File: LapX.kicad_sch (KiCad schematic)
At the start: 43 parts, among them J1 Conn_01x12, J2 Conn_02x01, J3 USB_C_Receptacle_PowerOnly_6P, J4 Micro_SD_Card_Det2, U2 TCMT4100

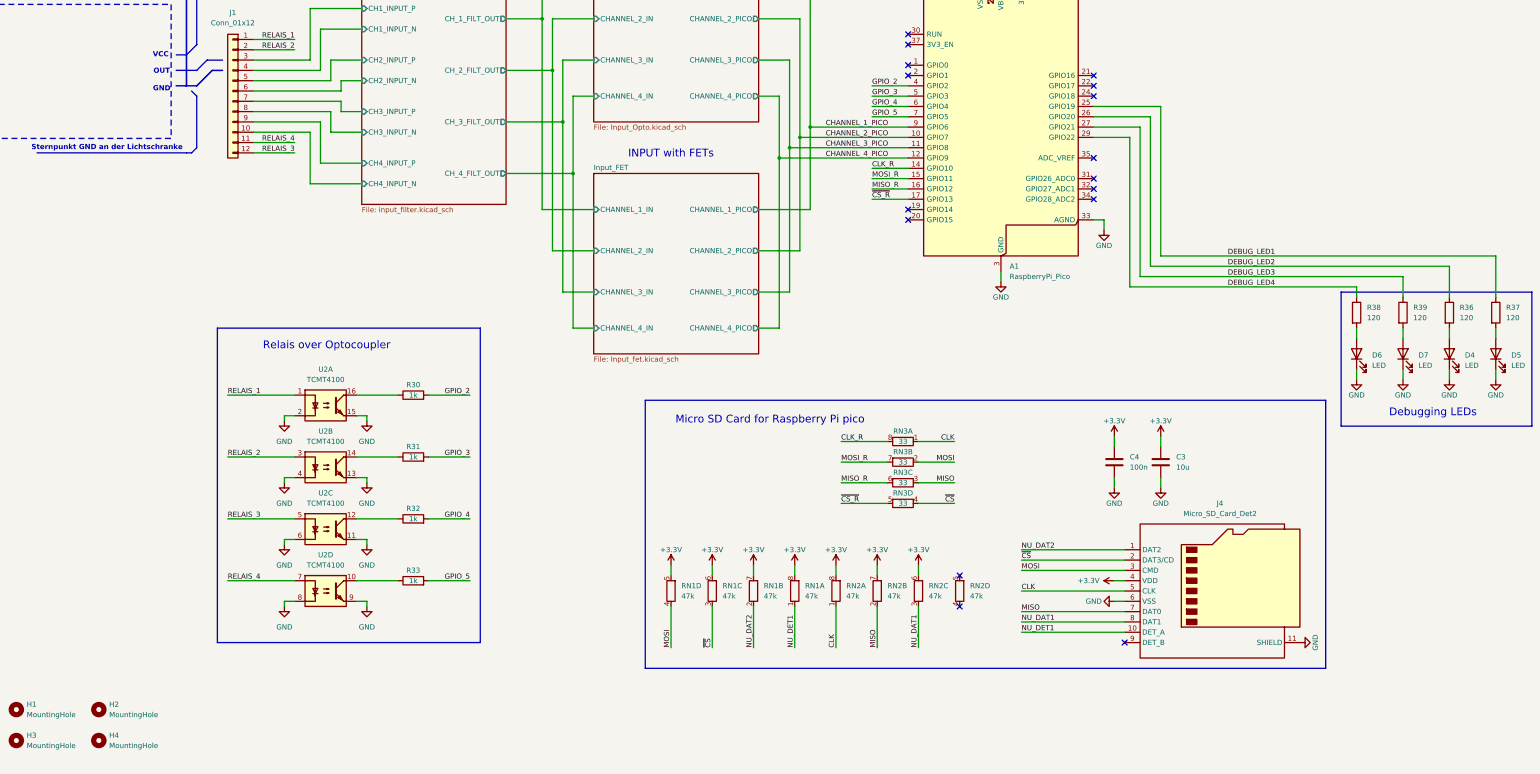
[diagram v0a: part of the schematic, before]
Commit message: Letzte Changes
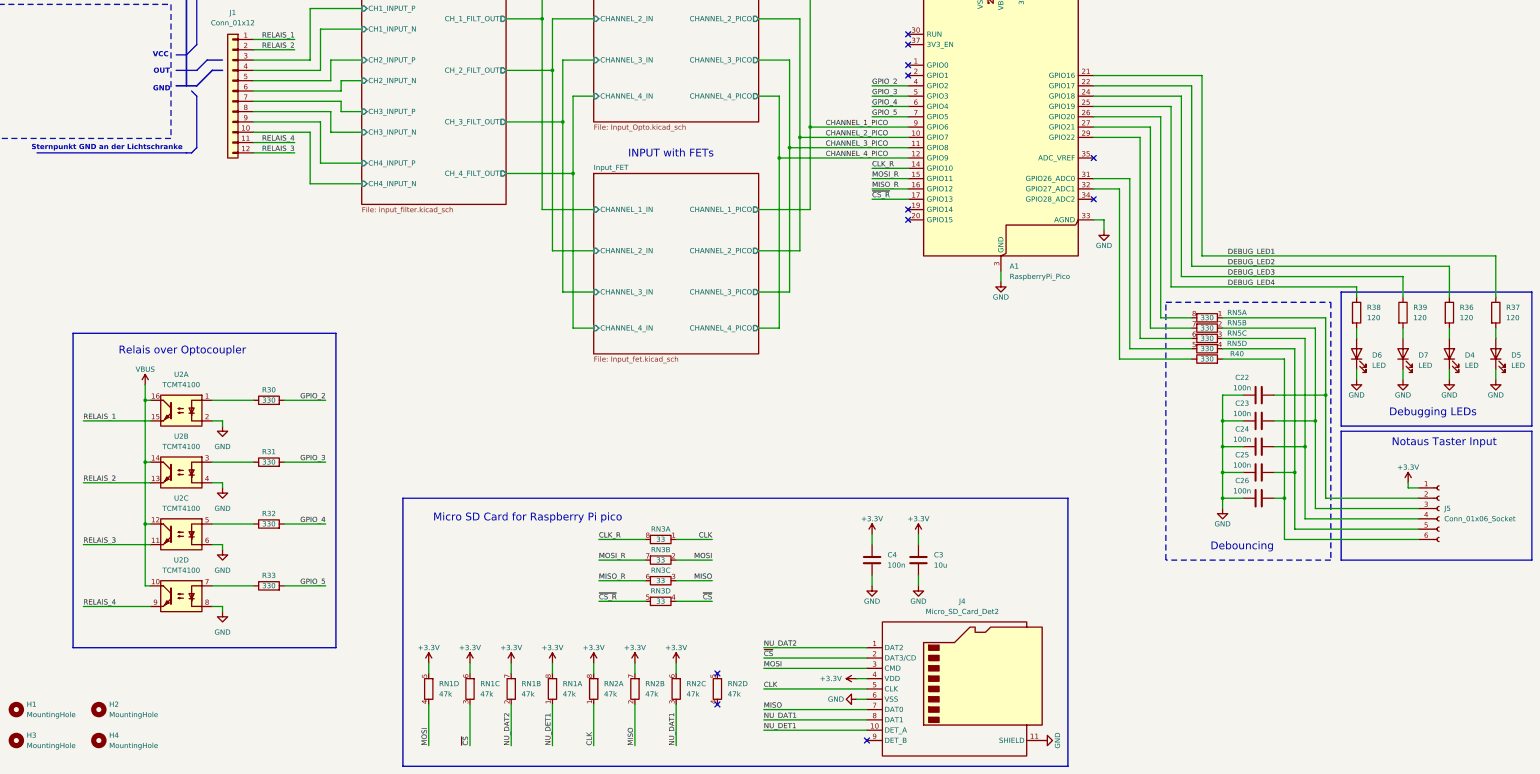
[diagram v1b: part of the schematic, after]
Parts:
- added C22, C23, C24, C25, C26: 100n, Capacitor_SMD:C_0603_1608Metric, symbol Device:C
- added J5: Conn_01x06_Socket, Connector_PinHeader_2.54mm:PinHeader_1x06_P2.54mm_Vertical, symbol Connector:Conn_01x06_Socket
- added R40: 330, Resistor_SMD:R_0603_1608Metric, symbol Device:R
- added RN5: 330, Resistor_SMD:R_Array_Convex_4x0603, symbol Device:R_Pack04_Split
- R30, R31, R32, R33: value 1k -> 330
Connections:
- net +3.3V: now also J5.1 (Pin_1)
- net DEBUG_LED1: now also A1.21 (GPIO16); no longer A1.25 (GPIO19)
- net DEBUG_LED2: now also A1.22 (GPIO17); no longer A1.26 (GPIO20)
- net DEBUG_LED3: now also A1.24 (GPIO18); no longer A1.27 (GPIO21)
- net DEBUG_LED4: now also A1.25 (GPIO19); no longer A1.29 (GPIO22)
- net GND: now also C22.1, C23.1, C24.1, C25.1, C26.1; no longer U2.11, U2.13, U2.15, U2.9
- net RELAIS_1: now also U2.15; no longer U2.1
- net RELAIS_2: now also U2.13; no longer U2.3
- net RELAIS_3: now also U2.11; no longer U2.5
- net RELAIS_4: now also U2.9; no longer U2.7
- net VBUS: now also U2.10, U2.12, U2.14, U2.16
- net at R33.1: now also U2.7; no longer U2.10
- net at R32.1: now also U2.5; no longer U2.12
- net at R30.1: now also U2.1; no longer U2.16
- net at R31.1: now also U2.3; no longer U2.14
- net at A1.31 (GPIO26_ADC0): now also RN5.5 (R4.2)
- net at A1.32 (GPIO27_ADC1): now also R40.1
- new net: C22.2, J5.2 (Pin_2), RN5.1 (R1.1)
- new net: A1.26 (GPIO20), RN5.8 (R1.2)
- new net: C24.2, J5.4 (Pin_4), RN5.3 (R3.1)
- new net: A1.29 (GPIO22), RN5.6 (R3.2)
- new net: C23.2, J5.3 (Pin_3), RN5.2 (R2.1)
- new net: A1.27 (GPIO21), RN5.7 (R2.2)
- new net: C25.2, J5.5 (Pin_5), RN5.4 (R4.1)
- new net: C26.2, J5.6 (Pin_6), R40.2
- no-connect marks 18 -> 13
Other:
- note added: "Debouncing"
- note added: "Notaus Taster Input"
- moved on the sheet: C3, C4, J4, R30, R31, R32, R33, RN1A, RN1B, RN1C, RN1D, RN2A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
